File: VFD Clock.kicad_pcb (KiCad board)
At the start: 2 copper layers, 224 x 78 mm, 37 parts, among them J2 Mode Button, J3 Up Button, J4 Down Button, J5 Select Button, U1 74HC595, U10 74HC595, U11 UDN2981A, U12 Minute Right, U13 74HC595, U14 UDN2981A, U15 Second Left, U16 74HC595, U17 UDN2981A, U18 Second Right, U19 XL6009 Module, U2 UDN2981A, U20 LM2596 Module, U21 DS3231 Module, U3 Hour Left, U4 74HC595, U5 UDN2981A, U6 Hour Right, U7 74HC595, U8 UDN2981A, U9 Minute Left

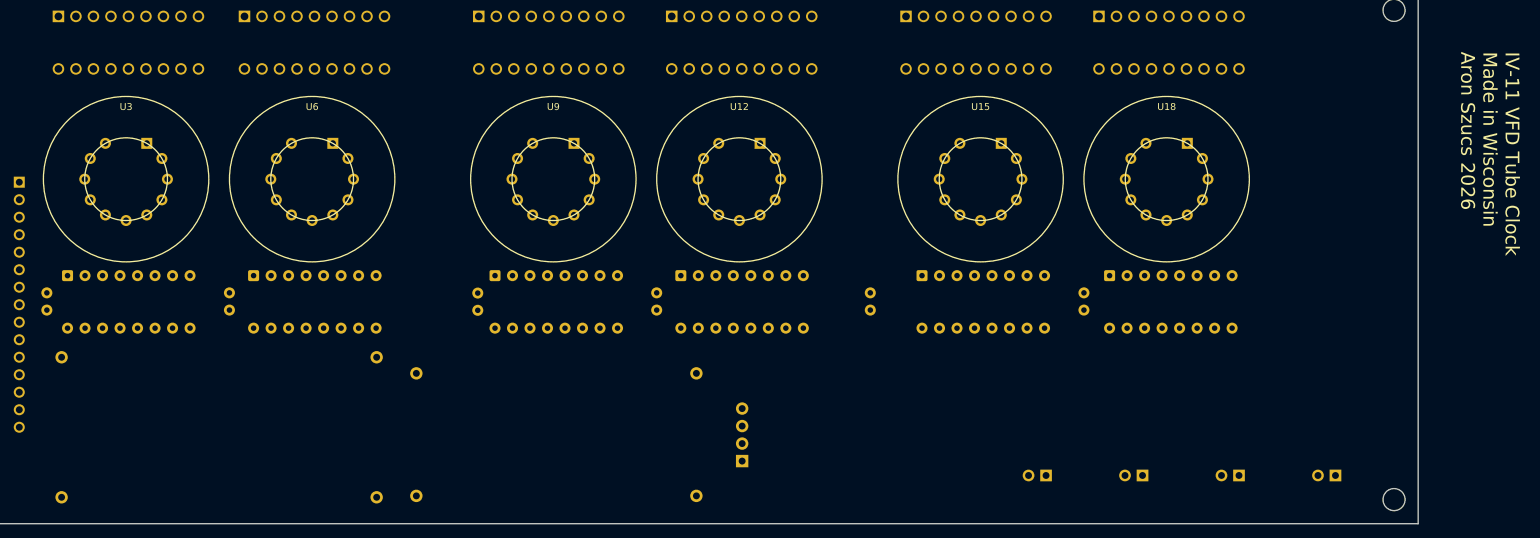
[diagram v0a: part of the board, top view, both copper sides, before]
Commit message: save
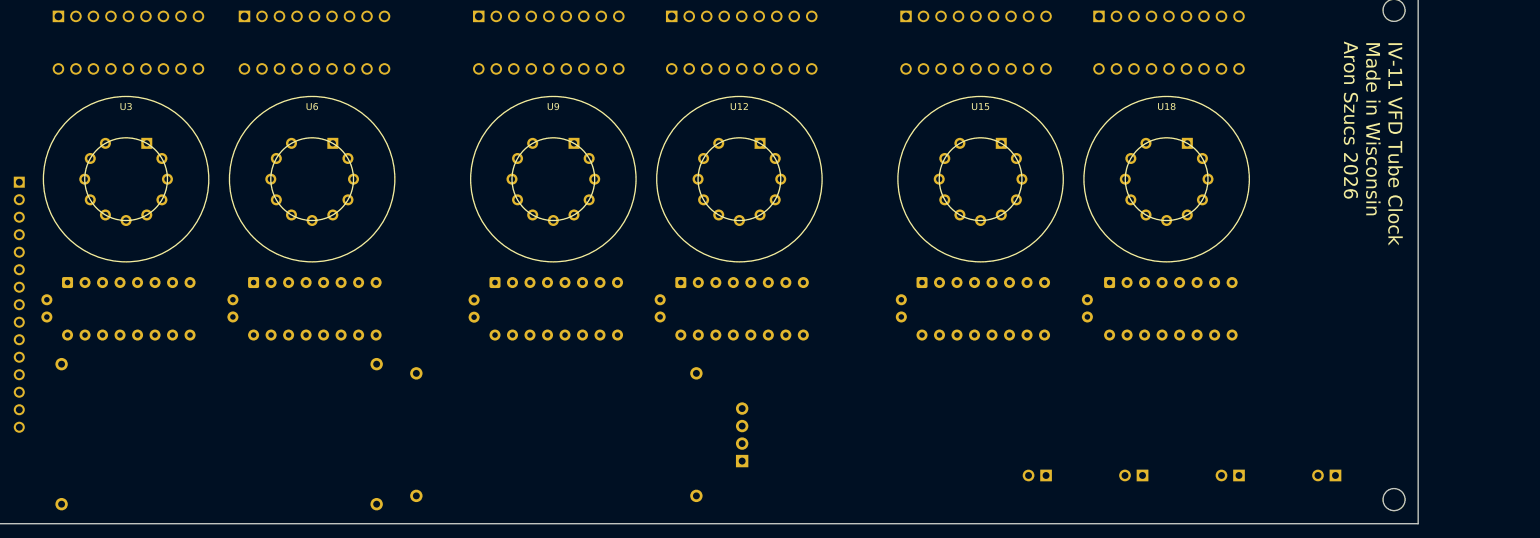
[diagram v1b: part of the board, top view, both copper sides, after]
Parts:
- moved C11 4.61 mm to (212.5, 120.0)
- moved C8 1.13 mm to (150.5, 120.0)
- moved C12 1.12 mm to (239.5, 120.0)
- moved C7 1.12 mm to (177.5, 120.0)
- moved C9 1.12 mm to (115.5, 120.0)
- moved C10 1.00 mm to (88.5, 120.0)
- moved U1 1.00 mm to (91.5, 115.0)
- moved U10 1.00 mm to (180.5, 115.0)
- moved U13 1.00 mm to (215.5, 115.0)
- moved U16 1.00 mm to (242.7, 115.0)
- moved U20 1.00 mm to (137.5, 125.5)
- moved U4 1.00 mm to (118.5, 115.0)
- moved U7 1.00 mm to (153.5, 115.0)
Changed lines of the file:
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@@
 	)
 	(setup
+		(stackup
+			(layer "F.SilkS"
+				(type "Top Silk Screen")
+			)
+			(layer "F.Paste"
+				(type "Top Solder Paste")
+			)
+			(layer "F.Mask"
+				(type "Top Solder Mask")
+				(thickness 0.01)
+			)
+			(layer "F.Cu"
+				(type "copper")
+				(thickness 0.035)
+			)
+			(layer "dielectric 1"
+				(type "core")
+				(thickness 1.51)
+				(material "FR4")
+				(epsilon_r 4.5)
+				(loss_tangent 0.02)
+			)
+			(layer "B.Cu"
+				(type "copper")
+				(thickness 0.035)
+			)
+			(layer "B.Mask"
+				(type "Bottom Solder Mask")
+				(thickness 0.01)
+			)
+			(layer "B.Paste"
+				(type "Bottom Solder Paste")
+			)
+			(layer "B.SilkS"
+				(type "Bottom Silk Screen")
+			)
+			(copper_finish "None")
+			(dielectric_constraints no)
+		)
 		(pad_to_mask_clearance 0)
 		(allow_soldermask_bridges_in_footprints no)
@@
 		(capping no)
 		(filling no)
+		(zone_defaults)
 		(grid_origin 175.5 100)
 		(pcbplotparams
@@
 	(footprint "Package_DIP:DIP-16_W7.62mm"
 		(layer "B.Cu")
-		(at 180.5 114 -90)
+		(at 180.5 115 -90)
 		(descr "16-lead though-hole mounted DIP package, row spacing 7.62mm (300 mils)")
 		(tags "THT DIP DIL PDIP 2.54mm 7.62mm 300mil")
@@
 		)
 		(point
-			(at 189.39 117.81)
+			(at 189.39 118.81)
 			(size 1.27)
 			(layer "B.Fab")
@@
 	(footprint "Package_DIP:DIP-16_W7.62mm"
 		(layer "B.Cu")
-		(at 118.5 114 -90)
+		(at 118.5 115 -90)
 		(descr "16-lead though-hole mounted DIP package, row spacing 7.62mm (300 mils)")
 		(tags "THT DIP DIL PDIP 2.54mm 7.62mm 300mil")
@@
 		)
 		(point
-			(at 127.39 117.81)
+			(at 127.39 118.81)
 			(size 1.27)
 			(layer "B.Fab")
@@
 	(footprint "Package_DIP:DIP-16_W7.62mm"
 		(layer "B.Cu")
-		(at 215.5 114 -90)
+		(at 215.5 115 -90)
 		(descr "16-lead though-hole mounted DIP package, row spacing 7.62mm (300 mils)")
 		(tags "THT DIP DIL PDIP 2.54mm 7.62mm 300mil")
@@
 		)
 		(point
-			(at 224.39 117.81)
+			(at 224.39 118.81)
 			(size 1.27)
 			(layer "B.Fab")
@@
 	(footprint "Package_DIP:DIP-16_W7.62mm"
 		(layer "B.Cu")
-		(at 91.5 114 -90)
+		(at 91.5 115 -90)
 		(descr "16-lead though-hole mounted DIP package, row spacing 7.62mm (300 mils)")
 		(tags "THT DIP DIL PDIP 2.54mm 7.62mm 300mil")
@@
 		)
 		(point
-			(at 100.39 117.81)
+			(at 100.39 118.81)
 			(size 1.27)
 			(layer "B.Fab")
@@
 	(footprint "Capacitor_THT:C_Disc_D3.0mm_W1.6mm_P2.50mm"
 		(layer "B.Cu")
-		(at 176.997842 118.997706 90)
+		(at 177.5 119.997706 90)
 		(descr "C, Disc series, Radial, pin pitch=2.50mm, diameter*width=3.0*1.6mm^2, Capacitor, http://www.vishay.com/docs/45233/krseries.pdf")
 		(tags "C Disc series Radial pin pitch 2.50mm diameter 3.0mm width 1.6mm Capacitor")
@@
 	(footprint "Custom Parts:LM2596 Module"
 		(layer "B.Cu")
-		(at 137.5 124.5047 180)
+		(at 137.5 125.5047 180)
 		(property "Reference" "U20"
 			(at 25.4 -8.66 0)
@@
 	(footprint "Capacitor_THT:C_Disc_D3.0mm_W1.6mm_P2.50mm"
 		(layer "B.Cu")
-		(at 151.031186 119.03105 90)
+		(at 150.5 120.03105 90)
 		(descr "C, Disc series, Radial, pin pitch=2.50mm, diameter*width=3.0*1.6mm^2, Capacitor, http://www.vishay.com/docs/45233/krseries.pdf")
 		(tags "C Disc series Radial pin pitch 2.50mm diameter 3.0mm width 1.6mm Capacitor")
@@
 	(footprint "Capacitor_THT:C_Disc_D3.0mm_W1.6mm_P2.50mm"
 		(layer "B.Cu")
-		(at 207.997842 118.997706 90)
+		(at 212.5 119.997706 90)
 		(descr "C, Disc series, Radial, pin pitch=2.50mm, diameter*width=3.0*1.6mm^2, Capacitor, http://www.vishay.com/docs/45233/krseries.pdf")
 		(tags "C Disc series Radial pin pitch 2.50mm diameter 3.0mm width 1.6mm Capacitor")
@@
 	(footprint "Capacitor_THT:C_Disc_D3.0mm_W1.6mm_P2.50mm"
 		(layer "B.Cu")
-		(at 238.997842 118.997706 90)
+		(at 239.5 119.997706 90)
 		(descr "C, Disc series, Radial, pin pitch=2.50mm, diameter*width=3.0*1.6mm^2, Capacitor, http://www.vishay.com/docs/45233/krseries.pdf")
 		(tags "C Disc series Radial pin pitch 2.50mm diameter 3.0mm width 1.6mm Capacitor")
@@
 	(footprint "Package_DIP:DIP-16_W7.62mm"
 		(layer "B.Cu")
-		(at 242.72 114 -90)
+		(at 242.72 115 -90)
 		(descr "16-lead though-hole mounted DIP package, row spacing 7.62mm (300 mils)")
 		(tags "THT DIP DIL PDIP 2.54mm 7.62mm 300mil")
@@
 		)
 		(point
-			(at 251.61 117.81)
+			(at 251.61 118.81)
 			(size 1.27)
 			(layer "B.Fab")
@@
 	(footprint "Capacitor_THT:C_Disc_D3.0mm_W1.6mm_P2.50mm"
 		(layer "B.Cu")
-		(at 114.997842 118.997706 90)
+		(at 115.5 119.997706 90)
 		(descr "C, Disc series, Radial, pin pitch=2.50mm, diameter*width=3.0*1.6mm^2, Capacitor, http://www.vishay.com/docs/45233/krseries.pdf")
 		(tags "C Disc series Radial pin pitch 2.50mm diameter 3.0mm width 1.6mm Capacitor")
@@
 	(footprint "Capacitor_THT:C_Disc_D3.0mm_W1.6mm_P2.50mm"
 		(layer "B.Cu")
-		(at 88.5 119 90)
+		(at 88.5 120 90)
 		(descr "C, Disc series, Radial, pin pitch=2.50mm, diameter*width=3.0*1.6mm^2, Capacitor, http://www.vishay.com/docs/45233/krseries.pdf")
 		(tags "C Disc series Radial pin pitch 2.50mm diameter 3.0mm width 1.6mm Capacitor")
@@
 		)
 		(property "Value" "100nF"
-			(at 5 1 180)
+			(at 6 0 90)
 			(layer "B.SilkS")
 			(effects
@@
 	(footprint "Package_DIP:DIP-16_W7.62mm"
 		(layer "B.Cu")
-		(at 153.533344 114 -90)
+		(at 153.533344 115 -90)
 		(descr "16-lead though-hole mounted DIP package, row spacing 7.62mm (300 mils)")
 		(tags "THT DIP DIL PDIP 2.54mm 7.62mm 300mil")
@@
 		)
 		(point
-			(at 162.423344 117.81)
+			(at 162.423344 118.81)
 			(size 1.27)
 			(layer "B.Fab")
@@
 	)
 	(gr_text "IV-11 VFD Tube Clock\nMade in Wisconsin\nAron Szucs 2026\n"
-		(at 293.5 81.5 270)
+		(at 276.5 80 270)
 		(layer "F.SilkS")
 		(effects
